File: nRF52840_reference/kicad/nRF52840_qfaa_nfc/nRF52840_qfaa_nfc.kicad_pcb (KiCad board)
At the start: 2 copper layers, 45 x 45 mm, 33 parts, among them J1 CONN_COAXIAL, U1 nRF52840, X1 XTAL_32MHZ, X2 XTAL_32KHZ

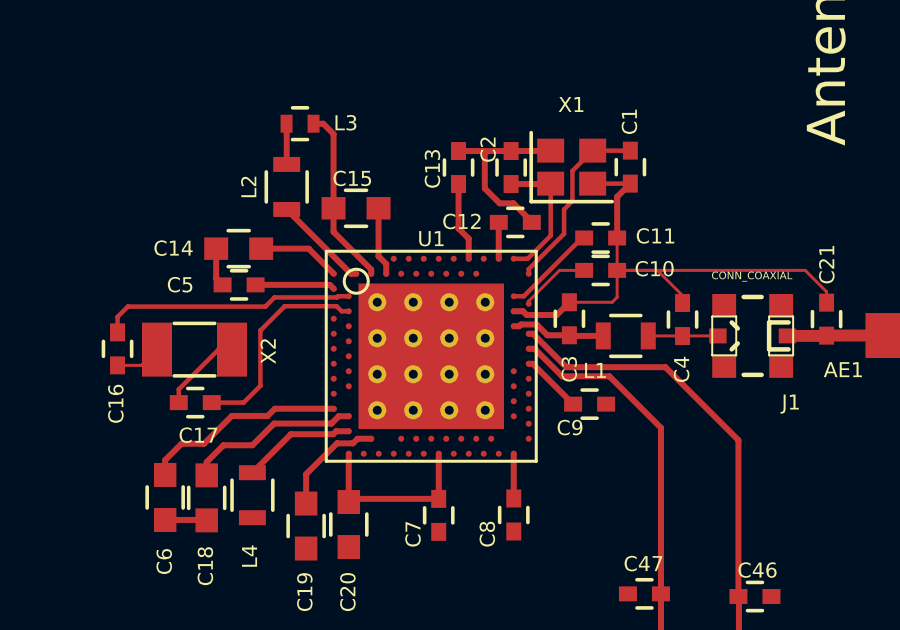
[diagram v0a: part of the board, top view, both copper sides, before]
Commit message: Update KiCAD Project nRF52840_qfaa_nfc
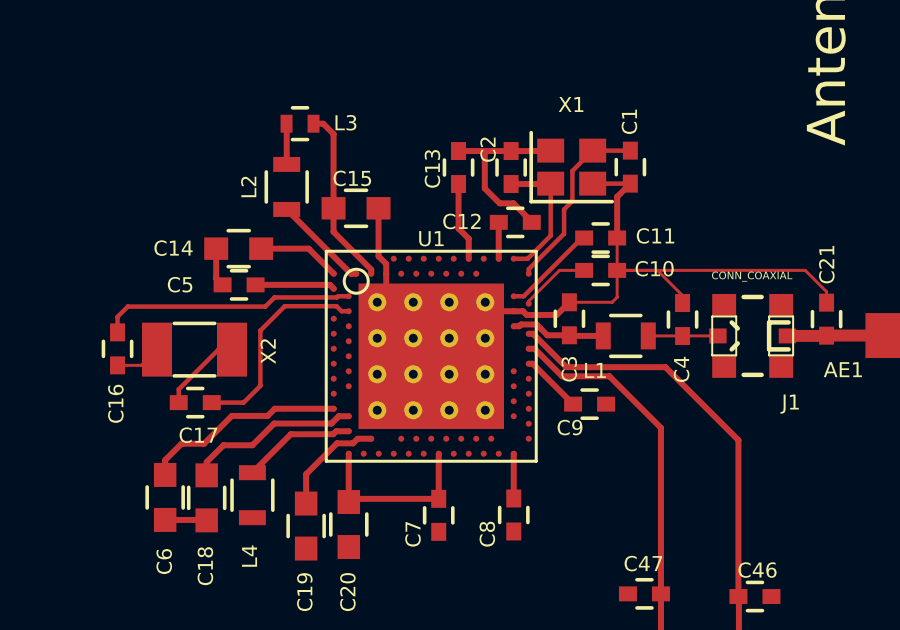
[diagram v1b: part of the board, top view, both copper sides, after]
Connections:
- U1 pad 74: Net-(U1-Pad74) -> GND
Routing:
- net GND: track 30.7 -> 37.5 mm
